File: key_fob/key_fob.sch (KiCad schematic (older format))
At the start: 20 parts, among them IC1 L4931ABDT33-TR, J1 Arduino-NANO-33, J2 B2B-PH-K-S_LF__SN_, U1 PS1240P02BT

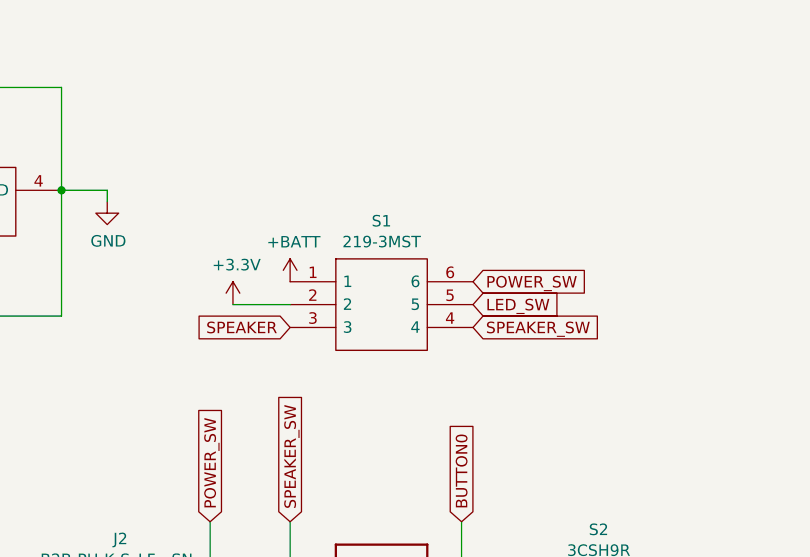
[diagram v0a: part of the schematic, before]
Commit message: Got some stuff started for key fod pcb
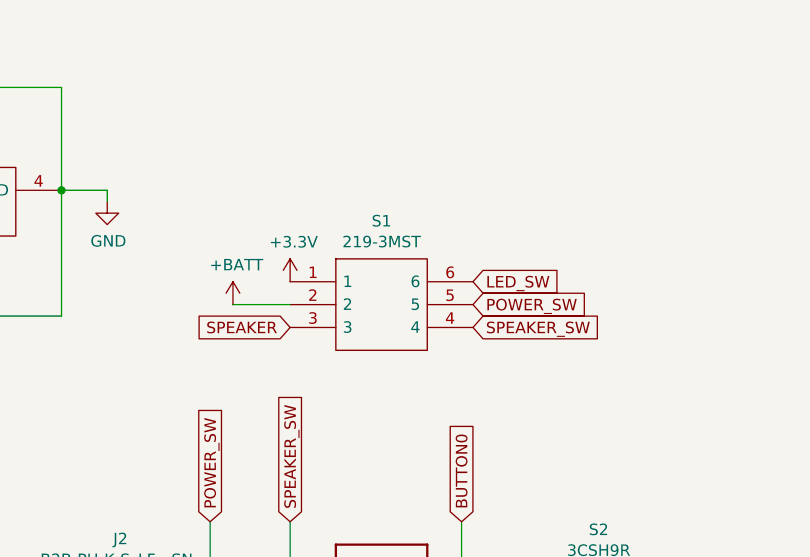
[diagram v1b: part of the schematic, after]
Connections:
- net +3V3: now also S1.1; no longer S1.2
- net +BATT: now also S1.2; no longer S1.1
- net LED_SW: now also S1.6; no longer S1.5
- net POWER_SW: now also S1.5; no longer S1.6
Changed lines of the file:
@@
 	7600 3550 7900 3550
-$Comp
-L power:+BATT #PWR0101
-U 1 1 5E36659B
-P 8250 2200
-F 0 "#PWR0101" H 8250 2050 50  0001 C CNN
-F 1 "+BATT" H 8265 2373 50  0000 C CNN
-F 2 "" H 8250 2200 50  0001 C CNN
-F 3 "" H 8250 2200 50  0001 C CNN
-	1    8250 2200
-	1    0    0    -1
-$EndComp
 $Comp
 L power:GND #PWR0102
@@
 F 3 "" H 7900 4100 50  0001 C CNN
 	1    7900 4100
-	1    0    0    -1
-$EndComp
-$Comp
-L power:+3.3V #PWR0103
-U 1 1 5E319CC0
-P 8000 2300
-F 0 "#PWR0103" H 8000 2150 50  0001 C CNN
-F 1 "+3.3V" H 8015 2473 50  0000 C CNN
-F 2 "" H 8000 2300 50  0001 C CNN
-F 3 "" H 8000 2300 50  0001 C CNN
-	1    8000 2300
 	1    0    0    -1
 $EndComp
@@
 Text GLabel 2750 3850 3    50   Input ~ 0
 POWER_LED
+Text GLabel 9050 2200 2    50   Input ~ 0
+LED_SW
 Text GLabel 9050 2300 2    50   Input ~ 0
-LED_SW
-Text GLabel 9050 2200 2    50   Input ~ 0
 POWER_SW
 Text GLabel 9050 2400 2    50   Input ~ 0
 SPEAKER_SW
-Wire Wire Line
-	8250 2300 8000 2300
 Text GLabel 4150 2850 1    50   Input ~ 0
 LED_SW
@@
 	1    0    0    -1
 $EndComp
+Wire Wire Line
+	8250 2300 8000 2300
+$Comp
+L power:+3.3V #PWR0103
+U 1 1 5E319CC0
+P 8250 2200
+F 0 "#PWR0103" H 8250 2050 50  0001 C CNN
+F 1 "+3.3V" H 8265 2373 50  0000 C CNN
+F 2 "" H 8250 2200 50  0001 C CNN
+F 3 "" H 8250 2200 50  0001 C CNN
+	1    8250 2200
+	1    0    0    -1
+$EndComp
+$Comp
+L power:+BATT #PWR?
+U 1 1 5E5C3234
+P 8000 2300
+F 0 "#PWR?" H 8000 2150 50  0001 C CNN
+F 1 "+BATT" H 8015 2473 50  0000 C CNN
+F 2 "" H 8000 2300 50  0001 C CNN
+F 3 "" H 8000 2300 50  0001 C CNN
+	1    8000 2300
+	1    0    0    -1
+$EndComp
